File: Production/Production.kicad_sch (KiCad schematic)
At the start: 28 parts, among them IC1 MAX3323EEPE+, IC2 AP7375-33SA-7, J1 530480510, J2 530480410, J3 USB4085-GF-A_REVB, U2 ADR02AUJZ-REEL7, U3 ATSAMD21G18A-AUT, Y1 32.768, 12.5pF

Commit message: Reloaded footprints & models after switching back to mac
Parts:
- C4: footprint Capacitor_SMD:C_0402_1005Metric -> Capacitor_SMD:C_0805_2012Metric
- J1: footprint Connector_Molex_2:Molex_PicoBlade_53048-0510_1x05_P1.25mm_Horizontal -> Connector_Molex:Molex_PicoBlade_53048-0510_1x05_P1.25mm_Horizontal
- J2: footprint Connector_Molex_2:Molex_PicoBlade_53048-0410_1x04_P1.25mm_Horizontal -> Connector_Molex:Molex_PicoBlade_53048-0410_1x04_P1.25mm_Horizontal
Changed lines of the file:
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@@
 		)
 		(instances
-			(project "Standalone"
+			(project "Production"
 				(path "/36880c03-5560-4777-bc12-f18c70ba2db4"
 					(reference "#PWR011")
@@
 		)
 		(instances
-			(project ""
+			(project "Production"
 				(path "/36880c03-5560-4777-bc12-f18c70ba2db4"
 					(reference "IC2")
@@
 		)
 		(instances
-			(project "Standalone"
+			(project "Production"
 				(path "/36880c03-5560-4777-bc12-f18c70ba2db4"
 					(reference "#PWR014")
@@
 			)
 		)
-		(property "Footprint" "Connector_Molex_2:Molex_PicoBlade_53048-0510_1x05_P1.25mm_Horizontal"
+		(property "Footprint" "Connector_Molex:Molex_PicoBlade_53048-0510_1x05_P1.25mm_Horizontal"
 			(at 54.61 54.61 0)
 			(effects
@@
 		)
 		(instances
-			(project "Standalone"
+			(project "Production"
 				(path "/36880c03-5560-4777-bc12-f18c70ba2db4"
 					(reference "J1")
@@
 		)
 		(instances
-			(project "Standalone"
+			(project "Production"
 				(path "/36880c03-5560-4777-bc12-f18c70ba2db4"
 					(reference "D4")
@@
 		)
 		(instances
-			(project "Standalone"
+			(project "Production"
 				(path "/36880c03-5560-4777-bc12-f18c70ba2db4"
 					(reference "#PWR018")
@@
 		)
 		(instances
-			(project "Standalone"
+			(project "Production"
 				(path "/36880c03-5560-4777-bc12-f18c70ba2db4"
 					(reference "#PWR08")
@@
 		)
 		(instances
-			(project "Standalone"
+			(project "Production"
 				(path "/36880c03-5560-4777-bc12-f18c70ba2db4"
 					(reference "#PWR03")
@@
 		)
 		(instances
-			(project "Standalone"
+			(project "Production"
 				(path "/36880c03-5560-4777-bc12-f18c70ba2db4"
 					(reference "C8")
@@
 		)
 		(instances
-			(project "Standalone"
+			(project "Production"
 				(path "/36880c03-5560-4777-bc12-f18c70ba2db4"
 					(reference "#PWR021")
@@
 		)
 		(instances
-			(project "Standalone"
+			(project "Production"
 				(path "/36880c03-5560-4777-bc12-f18c70ba2db4"
 					(reference "#PWR026")
@@
 		)
 		(instances
-			(project "Standalone"
+			(project "Production"
 				(path "/36880c03-5560-4777-bc12-f18c70ba2db4"
 					(reference "IC1")
@@
 		)
 		(instances
-			(project "Standalone"
+			(project "Production"
 				(path "/36880c03-5560-4777-bc12-f18c70ba2db4"
 					(reference "#PWR022")
@@
 		)
 		(instances
-			(project "Standalone"
+			(project "Production"
 				(path "/36880c03-5560-4777-bc12-f18c70ba2db4"
 					(reference "#PWR024")
@@
 		)
 		(instances
-			(project "Standalone"
+			(project "Production"
 				(path "/36880c03-5560-4777-bc12-f18c70ba2db4"
 					(reference "U2")
@@
 		)
 		(instances
-			(project "Standalone"
+			(project "Production"
 				(path "/36880c03-5560-4777-bc12-f18c70ba2db4"
 					(reference "#PWR016")
@@
 		)
 		(instances
-			(project "Standalone"
+			(project "Production"
 				(path "/36880c03-5560-4777-bc12-f18c70ba2db4"
 					(reference "C2")
@@
 		)
 		(instances
-			(project "Standalone"
+			(project "Production"
 				(path "/36880c03-5560-4777-bc12-f18c70ba2db4"
 					(reference "J3")
@@
 			)
 		)
-		(property "Footprint" "Capacitor_SMD:C_0402_1005Metric"
+		(property "Footprint" "Capacitor_SMD:C_0805_2012Metric"
 			(at 114.6048 39.37 0)
 			(effects
@@
 		)
 		(instances
-			(project "Standalone"
+			(project "Production"
 				(path "/36880c03-5560-4777-bc12-f18c70ba2db4"
 					(reference "C4")
@@
 		)
 		(instances
-			(project "Standalone"
+			(project "Production"
 				(path "/36880c03-5560-4777-bc12-f18c70ba2db4"
 					(reference "R2")
@@
 		)
 		(instances
-			(project "Standalone"
+			(project "Production"
 				(path "/36880c03-5560-4777-bc12-f18c70ba2db4"
 					(reference "#PWR039")
@@
 		)
 		(instances
-			(project "Standalone"
+			(project "Production"
 				(path "/36880c03-5560-4777-bc12-f18c70ba2db4"
 					(reference "#PWR013")
@@
 		)
 		(instances
-			(project "Standalone"
+			(project "Production"
 				(path "/36880c03-5560-4777-bc12-f18c70ba2db4"
 					(reference "D1")
@@
 		)
 		(instances
-			(project "Standalone"
+			(project "Production"
 				(path "/36880c03-5560-4777-bc12-f18c70ba2db4"
 					(reference "#PWR06")
@@
 		)
 		(instances
-			(project "Standalone"
+			(project "Production"
 				(path "/36880c03-5560-4777-bc12-f18c70ba2db4"
 					(reference "#PWR07")
@@
 		)
 		(instances
-			(project "Standalone"
+			(project "Production"
 				(path "/36880c03-5560-4777-bc12-f18c70ba2db4"
 					(reference "D2")
@@
 		)
 		(instances
-			(project "Standalone"
+			(project "Production"
 				(path "/36880c03-5560-4777-bc12-f18c70ba2db4"
 					(reference "#PWR015")
@@
 		)
 		(instances
-			(project "Standalone"
+			(project "Production"
 				(path "/36880c03-5560-4777-bc12-f18c70ba2db4"
 					(reference "#PWR020")
@@
 		)
 		(instances
-			(project "Standalone"
+			(project "Production"
 				(path "/36880c03-5560-4777-bc12-f18c70ba2db4"
 					(reference "#PWR017")
@@
 		)
 		(instances
-			(project "Standalone"
+			(project "Production"
 				(path "/36880c03-5560-4777-bc12-f18c70ba2db4"
 					(reference "R1")
@@
 		)
 		(instances
-			(project ""
+			(project "Production"
 				(path "/36880c03-5560-4777-bc12-f18c70ba2db4"
 					(reference "S1")
@@
 		)
 		(instances
-			(project "Standalone"
+			(project "Production"
 				(path "/36880c03-5560-4777-bc12-f18c70ba2db4"
 					(reference "#PWR02")
@@
 		)
 		(instances
-			(project "Standalone"
+			(project "Production"
 				(path "/36880c03-5560-4777-bc12-f18c70ba2db4"
 					(reference "#PWR04")
@@
 		)
 		(instances
-			(project "Standalone"
+			(project "Production"
 				(path "/36880c03-5560-4777-bc12-f18c70ba2db4"
 					(reference "R8")
@@
 		)
 		(instances
-			(project "Standalone"
+			(project "Production"
 				(path "/36880c03-5560-4777-bc12-f18c70ba2db4"
 					(reference "C5")
@@
 		)
 		(instances
-			(project ""
+			(project "Production"
 				(path "/36880c03-5560-4777-bc12-f18c70ba2db4"
 					(reference "RESET1")
@@
 		)
 		(instances
-			(project "Standalone"
+			(project "Production"
 				(path "/36880c03-5560-4777-bc12-f18c70ba2db4"
 					(reference "C1")
@@
 		)
 		(instances
-			(project "Standalone"
+			(project "Production"
 				(path "/36880c03-5560-4777-bc12-f18c70ba2db4"
 					(reference "#PWR01")
@@
 		)
 		(instances
-			(project "Standalone"
+			(project "Production"
 				(path "/36880c03-5560-4777-bc12-f18c70ba2db4"
 					(reference "R3")
@@
 		)
 		(instances
-			(project "Standalone"
+			(project "Production"
 				(path "/36880c03-5560-4777-bc12-f18c70ba2db4"
 					(reference "#PWR010")
@@
 		)
 		(instances
-			(project "Standalone"
+			(project "Production"
 				(path "/36880c03-5560-4777-bc12-f18c70ba2db4"
 					(reference "R5")
@@
 		)
 		(instances
-			(project "Standalone"
+			(project "Production"
 				(path "/36880c03-5560-4777-bc12-f18c70ba2db4"
 					(reference "C6")
@@
 		)
 		(instances
-			(project "Standalone"
+			(project "Production"
 				(path "/36880c03-5560-4777-bc12-f18c70ba2db4"
 					(reference "C7")
@@
 		)
 		(instances
-			(project "Standalone"
+			(project "Production"
 				(path "/36880c03-5560-4777-bc12-f18c70ba2db4"
 					(reference "U3")
@@
 		)
 		(instances
-			(project "Standalone"
+			(project "Production"
 				(path "/36880c03-5560-4777-bc12-f18c70ba2db4"
 					(reference "Y1")
@@
 		)
 		(instances
-			(project "Standalone"
+			(project "Production"
 				(path "/36880c03-5560-4777-bc12-f18c70ba2db4"
 					(reference "#PWR023")
@@
 		)
 		(instances
-			(project "Standalone"
+			(project "Production"
 				(path "/36880c03-5560-4777-bc12-f18c70ba2db4"
 					(reference "#PWR09")
@@
 		)
 		(instances
-			(project "Standalone"
+			(project "Production"
 				(path "/36880c03-5560-4777-bc12-f18c70ba2db4"
 					(reference "#PWR012")
@@
 			)
 		)
-		(property "Footprint" "Connector_Molex_2:Molex_PicoBlade_53048-0410_1x04_P1.25mm_Horizontal"
+		(property "Footprint" "Connector_Molex:Molex_PicoBlade_53048-0410_1x04_P1.25mm_Horizontal"
 			(at 54.61 81.28 0)
 			(effects
@@
 		)
 		(instances
-			(project "Standalone"
+			(project "Production"
 				(path "/36880c03-5560-4777-bc12-f18c70ba2db4"
 					(reference "J2")
@@
 		)
 		(instances
-			(project "Standalone"
+			(project "Production"
 				(path "/36880c03-5560-4777-bc12-f18c70ba2db4"
 					(reference "#PWR05")
@@
 		)
 		(instances
-			(project "Standalone"
+			(project "Production"
 				(path "/36880c03-5560-4777-bc12-f18c70ba2db4"
 					(reference "C3")
@@
 		)
 		(instances
-			(project "Standalone"
+			(project "Production"
 				(path "/36880c03-5560-4777-bc12-f18c70ba2db4"
 					(reference "#PWR025")

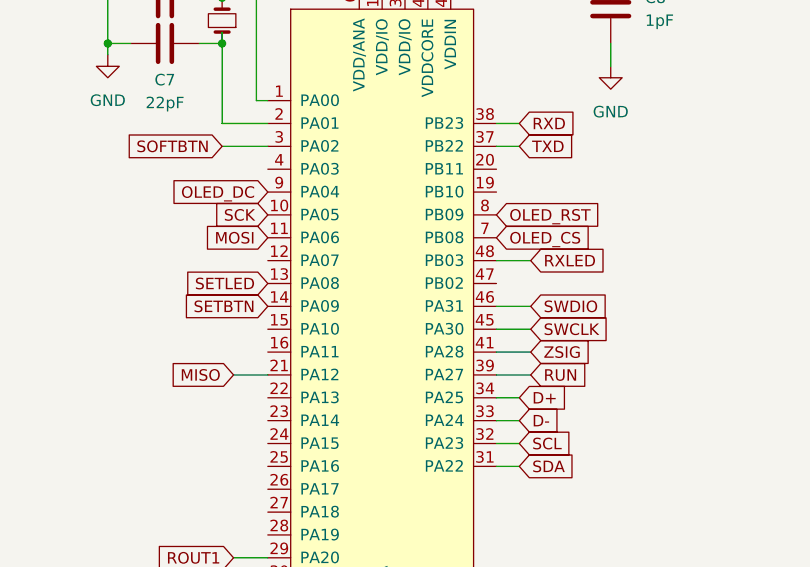
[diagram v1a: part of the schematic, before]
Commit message: v1, as submitted for production
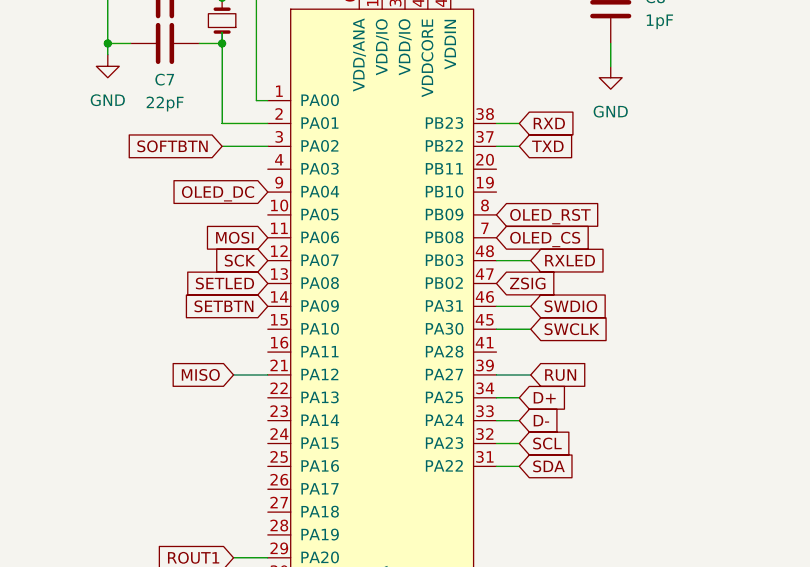
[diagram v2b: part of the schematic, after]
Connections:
- net SCK: now also U3.12 (PA07); no longer U3.10 (PA05)
- net ZSIG: now also U3.47 (PB02); no longer U3.41 (PA28)
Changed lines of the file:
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@@
-	(wire
-		(pts
-			(xy 256.54 104.14) (xy 260.35 104.14)
-		)
-		(stroke
-			(width 0)
-			(type default)
-		)
-	)
 	(wire
 		(pts
@@
 	(global_label "SCK"
 		(shape input)
-		(at 231.14 88.9 180)
+		(at 231.14 93.98 180)
 		(fields_autoplaced yes)
 		(effects
@@
 		)
 		(property "Intersheetrefs" "${INTERSHEET_REFS}"
-			(at 224.4053 88.9 0)
+			(at 224.4053 93.98 0)
 			(effects
 				(font
@@
 	(global_label "ZSIG"
 		(shape input)
-		(at 260.35 104.14 0)
+		(at 256.54 96.52 0)
 		(fields_autoplaced yes)
 		(effects
@@
 		)
 		(property "Intersheetrefs" "${INTERSHEET_REFS}"
-			(at 267.629 104.14 0)
-			(effects
-				(font
+			(at 263.819 96.52 0)
+			(effects
+				(font
